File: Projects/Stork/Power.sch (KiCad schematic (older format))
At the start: 18 parts, among them J25 Conn_02x03_Odd_Even, J26 Conn_01x03_Male, J28 Conn_01x03_Male, J29 Conn_01x03_Male, J30 Conn_01x03_Male, U50 TPS79330-EP, U51 TPS73150DBV

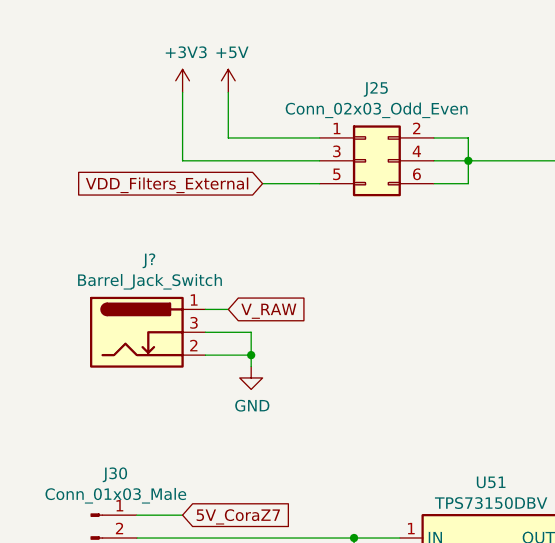
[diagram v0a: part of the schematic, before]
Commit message: added logo
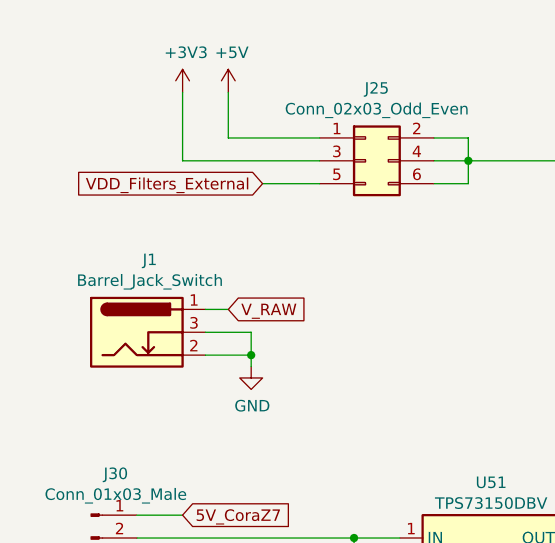
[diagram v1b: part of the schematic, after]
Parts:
- gave numbers to parts that had none: 1
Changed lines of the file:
@@
 $EndComp
 $Comp
-L Connector:Barrel_Jack_Switch J?
+L Connector:Barrel_Jack_Switch J1
 U 1 1 5EA23779
 P 1050 2200
-F 0 "J?" H 1107 2517 50  0000 C CNN
+F 0 "J1" H 1107 2517 50  0000 C CNN
 F 1 "Barrel_Jack_Switch" H 1107 2426 50  0000 C CNN
 F 2 "footprint:FC681465P" H 1100 2160 50  0001 C CNN
@@
 $EndComp
 $Comp
-L power:GND #PWR?
+L power:GND #PWR0152
 U 1 1 5EA2418A
 P 1550 2350
-F 0 "#PWR?" H 1550 2100 50  0001 C CNN
+F 0 "#PWR0152" H 1550 2100 50  0001 C CNN
 F 1 "GND" H 1555 2177 50  0000 C CNN
 F 2 "" H 1550 2350 50  0001 C CNN
